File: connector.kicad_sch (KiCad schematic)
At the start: 29 parts, among them J1 Conn_01x04, J10 Conn_02x02_Counter_Clockwise, J11 Conn_02x02_Counter_Clockwise, J12 Conn_02x02_Counter_Clockwise, J13 Conn_02x02_Counter_Clockwise, J14 Conn_02x02_Counter_Clockwise, J15 Conn_01x02, J16 Conn_01x02, J17 Conn_01x02, J18 Conn_01x02, J19 Conn_01x01, J20 Conn_01x01, J21 Conn_01x01, J22 Conn_01x01, J23 Conn_01x02, J24 Conn_01x02, J25 Conn_01x08, J26 Conn_01x08, J27 Conn_01x04, J3 Conn_01x04, J5 Conn_01x04, J7 Conn_02x02_Counter_Clockwise, J8 Conn_02x02_Counter_Clockwise, J9 Conn_02x02_Counter_Clockwise, P1 USB_C_Plug_USB2.0

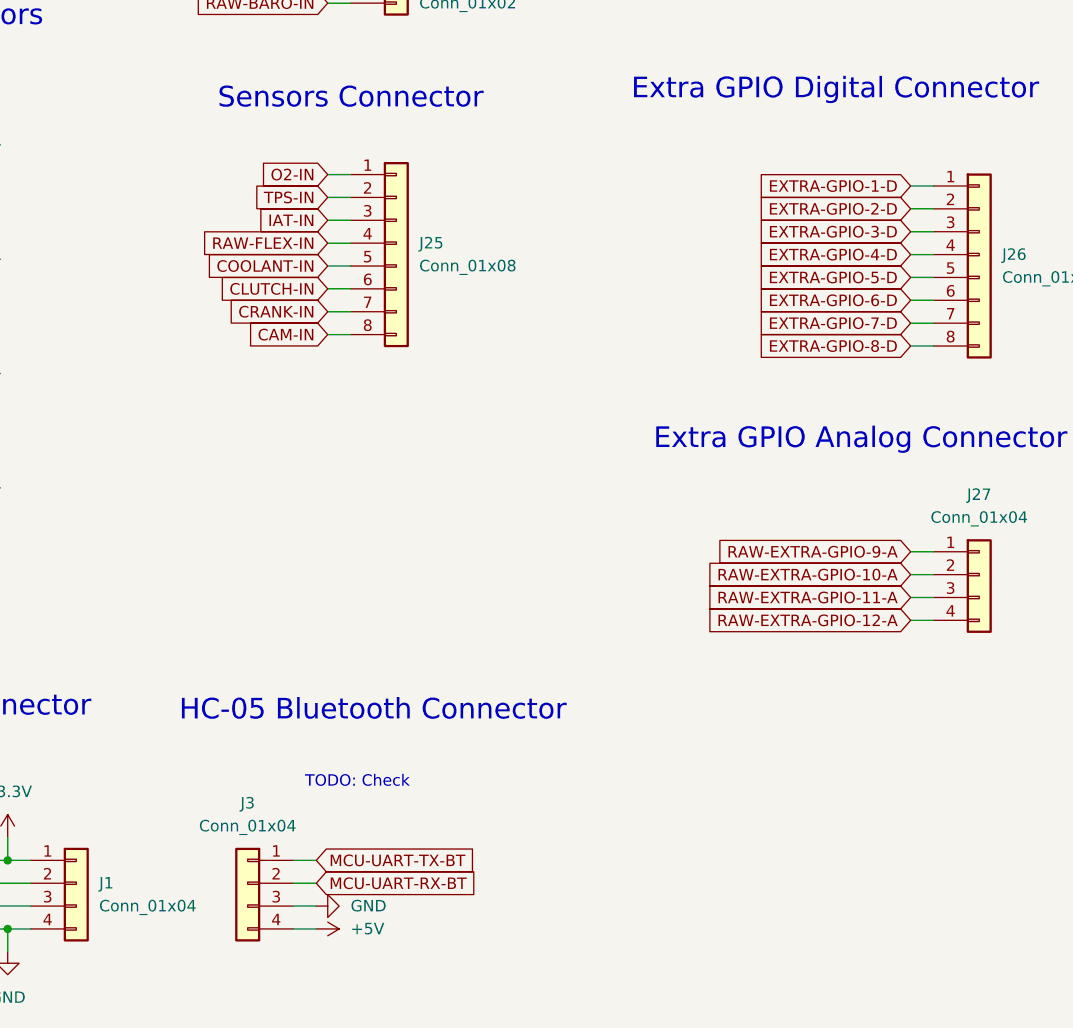
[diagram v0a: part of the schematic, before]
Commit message: Pre MCU switch
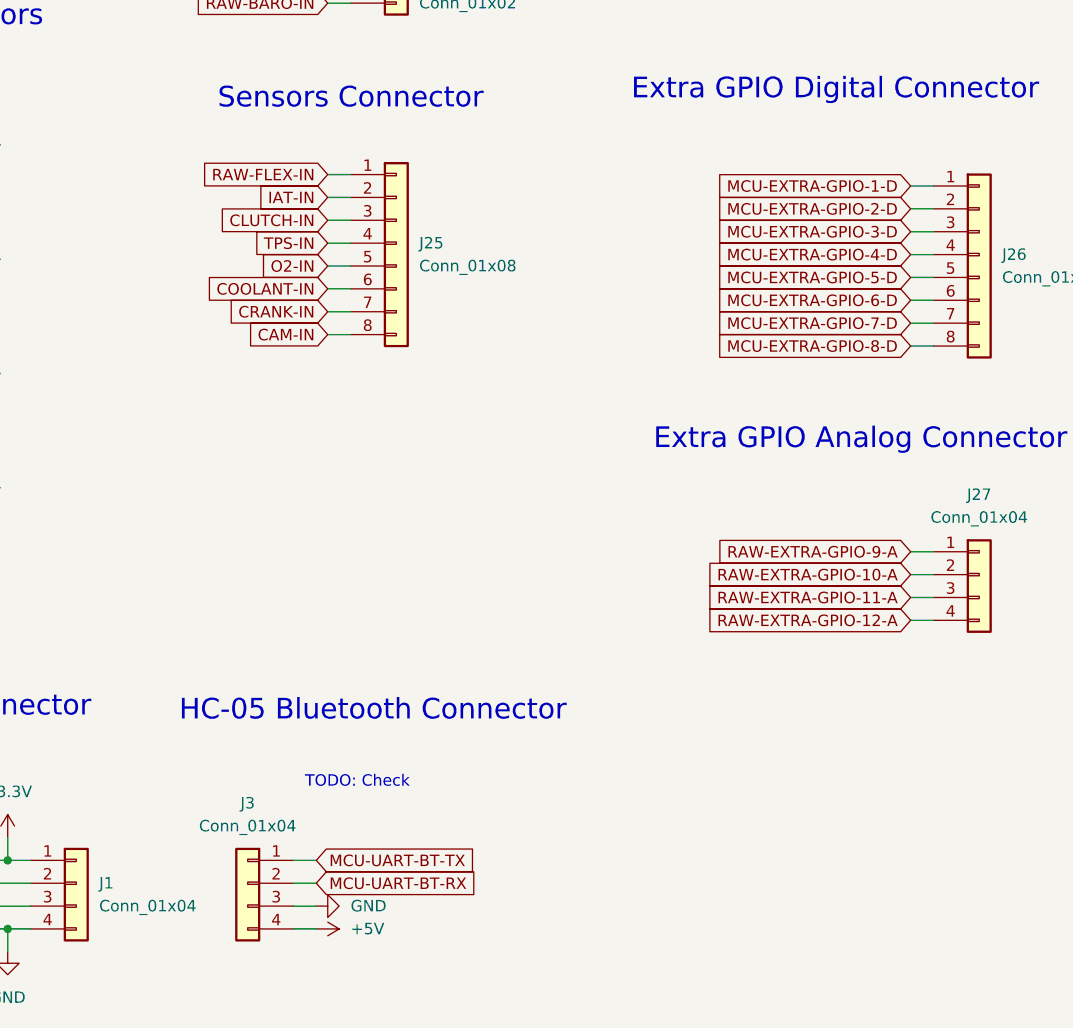
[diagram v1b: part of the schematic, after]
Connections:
- net CLUTCH-IN: now also J25.3 (Pin_3); no longer J25.6 (Pin_6)
- net COOLANT-IN: now also J25.6 (Pin_6); no longer J25.5 (Pin_5)
- net IAT-IN: now also J25.2 (Pin_2); no longer J25.3 (Pin_3)
- net O2-IN: now also J25.5 (Pin_5); no longer J25.1 (Pin_1)
- net RAW-FLEX-IN: now also J25.1 (Pin_1); no longer J25.4 (Pin_4)
- net TPS-IN: now also J25.4 (Pin_4); no longer J25.2 (Pin_2)
- net EXTRA-GPIO-1-D renamed MCU-EXTRA-GPIO-1-D
- net EXTRA-GPIO-2-D renamed MCU-EXTRA-GPIO-2-D
- net EXTRA-GPIO-3-D renamed MCU-EXTRA-GPIO-3-D
- net EXTRA-GPIO-4-D renamed MCU-EXTRA-GPIO-4-D
- net EXTRA-GPIO-5-D renamed MCU-EXTRA-GPIO-5-D
- net EXTRA-GPIO-6-D renamed MCU-EXTRA-GPIO-6-D
- net EXTRA-GPIO-7-D renamed MCU-EXTRA-GPIO-7-D
- net EXTRA-GPIO-8-D renamed MCU-EXTRA-GPIO-8-D
- net MCU-UART-RX-BT renamed MCU-UART-BT-RX
- net MCU-UART-TX-BT renamed MCU-UART-BT-TX
